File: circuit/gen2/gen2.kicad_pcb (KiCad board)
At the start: 2 copper layers, 100 x 88.9 mm, 5 parts

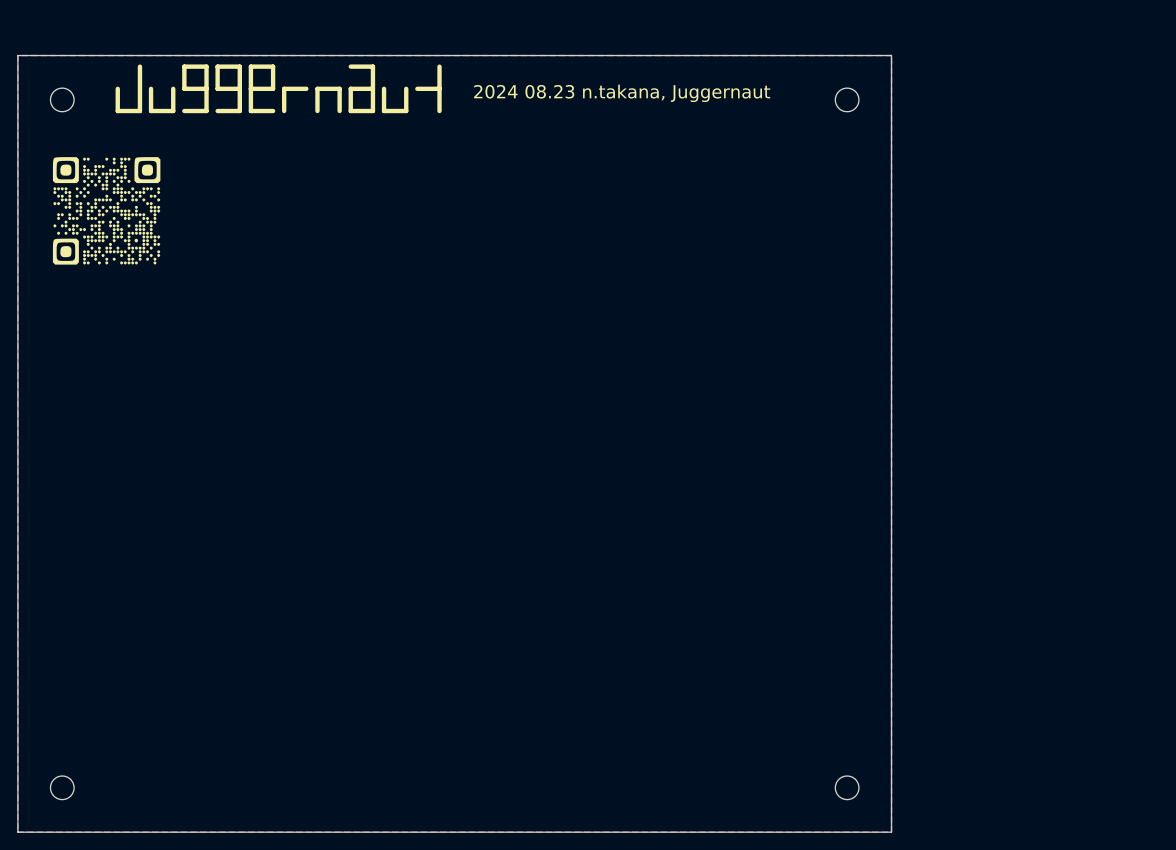
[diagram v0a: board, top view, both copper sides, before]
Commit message: [update] gen2 is production ready
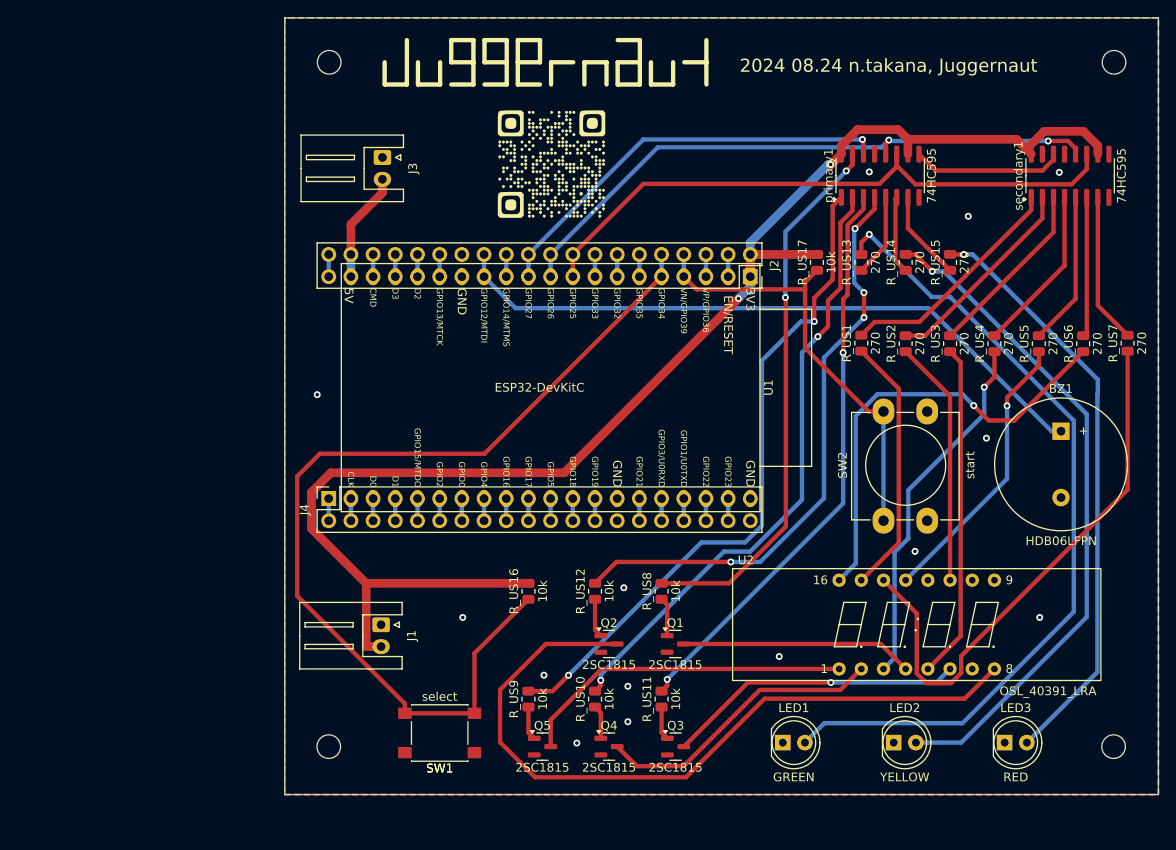
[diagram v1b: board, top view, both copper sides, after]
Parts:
- added BZ1: HDB06LFPN, Buzzer_Beeper:Buzzer_15x7.5RM7.6, F.Cu at (195.6, 106.5)
- added J1: Conn_01x02_Socket, Connector_JST:JST_XH_S2B-XH-A_1x02_P2.50mm_Horizontal, F.Cu at (117.8, 128.7)
- added J2: Conn_02x20_Row_Letter_Last, MyPartsLibrary:PinSocket_2x20_P2.54mm_1a-19a, F.Cu at (160.0, 88.8)
- added J3: Conn_01x02_Socket, Connector_JST:JST_XH_S2B-XH-A_1x02_P2.50mm_Horizontal, F.Cu at (117.9, 75.2)
- added J4: Conn_02x20_Row_Letter_Last, MyPartsLibrary:PinSocket_2x20_P2.54mm_20a_38a, F.Cu at (111.8, 114.2)
- added LED1: GREEN, LED_THT:LED_D5.0mm, F.Cu at (163.7, 142.1)
- added LED2: YELLOW, LED_THT:LED_D5.0mm, F.Cu at (176.4, 142.1)
- added LED3: RED, LED_THT:LED_D5.0mm, F.Cu at (189.1, 142.1)
- added Q1: 2SC1815, Package_TO_SOT_SMD:SOT-23, F.Cu at (151.5, 130.9)
- added Q2: 2SC1815, Package_TO_SOT_SMD:SOT-23, F.Cu at (143.9, 130.9)
- added Q3: 2SC1815, Package_TO_SOT_SMD:SOT-23, F.Cu at (151.5, 142.6)
- added Q4: 2SC1815, Package_TO_SOT_SMD:SOT-23, F.Cu at (143.9, 142.6)
- added Q5: 2SC1815, Package_TO_SOT_SMD:SOT-23, F.Cu at (136.2, 142.6)
- added R_US1: 270, Resistor_SMD:R_0805_2012Metric, F.Cu at (172.7, 96.4)
- added R_US10: 10k, Resistor_SMD:R_0805_2012Metric, F.Cu at (142.3, 137.2)
- added R_US11: 10k, Resistor_SMD:R_0805_2012Metric, F.Cu at (149.9, 137.2)
- added R_US12: 10k, Resistor_SMD:R_0805_2012Metric, F.Cu at (142.3, 124.8)
- added R_US13: 270, Resistor_SMD:R_0805_2012Metric, F.Cu at (172.7, 87.2)
- added R_US14: 270, Resistor_SMD:R_0805_2012Metric, F.Cu at (177.8, 87.2)
- added R_US15: 270, Resistor_SMD:R_0805_2012Metric, F.Cu at (182.9, 87.2)
- added R_US16: 10k, Resistor_SMD:R_0805_2012Metric, F.Cu at (134.6, 124.8)
- added R_US17: 10k, Resistor_SMD:R_0805_2012Metric, F.Cu at (167.7, 87.2)
- added R_US2: 270, Resistor_SMD:R_0805_2012Metric, F.Cu at (177.8, 96.5)
- added R_US3: 270, Resistor_SMD:R_0805_2012Metric, F.Cu at (182.9, 96.5)
- added R_US4: 270, Resistor_SMD:R_0805_2012Metric, F.Cu at (188.0, 96.5)
- added R_US5: 270, Resistor_SMD:R_0805_2012Metric, F.Cu at (193.1, 96.5)
- added R_US6: 270, Resistor_SMD:R_0805_2012Metric, F.Cu at (198.1, 96.5)
- added R_US7: 270, Resistor_SMD:R_0805_2012Metric, F.Cu at (203.2, 96.4)
- added R_US8: 10k, Resistor_SMD:R_0805_2012Metric, F.Cu at (149.9, 124.8)
- added R_US9: 10k, Resistor_SMD:R_0805_2012Metric, F.Cu at (134.6, 137.2)
- added SW1: select, Button_Switch_SMD:SW_SPST_PTS645, F.Cu at (124.5, 141.0)
- added SW2: start, Button_Switch_THT:SW_PUSH-12mm_Wuerth-430476085716, F.Cu at (175.3, 116.7)
- added U1: ESP32-DevKitC, MyPartsLibrary:ESP32-DevKitC, F.Cu at (160.0, 88.8)
- added U2: OSL_40391_LRA, MyPartsLibrary:OSL_40391_LRA, F.Cu at (179.1, 128.6)
- added primary1: 74HC595, Package_SO:SOIC-16_3.9x9.9mm_P1.27mm, F.Cu at (174.9, 77.3)
- added secondary1: 74HC595, Package_SO:SOIC-16_3.9x9.9mm_P1.27mm, F.Cu at (196.6, 77.3)
- moved G*** 51.2 mm to (137.3, 75.9)
- moved hole_lower_left 30.9 mm to (111.8, 142.6)
- moved hole_lower_right 30.9 mm to (201.6, 142.6)
- moved hole_upper_left 30.9 mm to (111.8, 64.3)
- moved hole_upper_right 30.9 mm to (201.7, 64.3)
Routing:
- net +3V3: track 0.00 -> 165.0 mm, vias 0 -> 2
- net /Pin5: track 0.00 -> 109.8 mm
- net Net-(LED1-A): track 0.00 -> 93.8 mm, vias 0 -> 1
- net Net-(Q2-C): track 0.00 -> 85.0 mm
- net Net-(LED2-A): track 0.00 -> 77.0 mm, vias 0 -> 1
- net Net-(primary1-QB): track 0.00 -> 76.8 mm, vias 0 -> 2
- net /Pin13: track 0.00 -> 75.9 mm
- net /Pin9: track 0.00 -> 71.0 mm
- net /Pin10: track 0.00 -> 70.9 mm, vias 0 -> 2
- net Net-(primary1-QC): track 0.00 -> 70.5 mm, vias 0 -> 2
- net Net-(primary1-QE): track 0.00 -> 68.0 mm, vias 0 -> 4
- net Net-(LED3-A): track 0.00 -> 67.8 mm, vias 0 -> 1
- net Net-(primary1-QD): track 0.00 -> 66.1 mm, vias 0 -> 2
- net Net-(U2-a/D1): track 0.00 -> 63.0 mm
- net Net-(primary1-QA): track 0.00 -> 62.7 mm, vias 0 -> 2
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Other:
- board text added: "2024 08.24 n.takana, Juggernaut"
- board text removed: "2024 08.23 n.takana, Juggernaut"
